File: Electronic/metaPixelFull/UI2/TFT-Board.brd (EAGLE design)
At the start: 56 x 60 mm, 28 parts, among them IC1 74HCT14N, IC2 74HCT14N

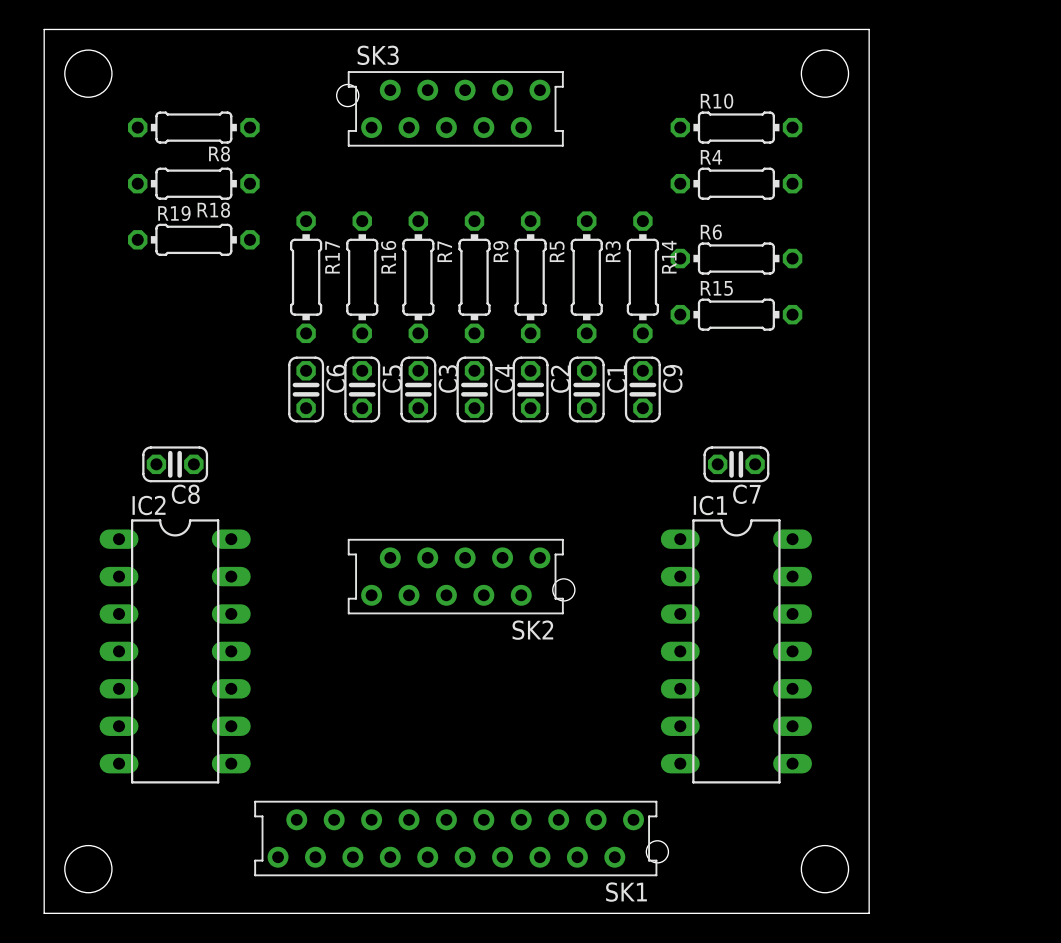
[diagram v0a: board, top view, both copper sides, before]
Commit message: rework UI
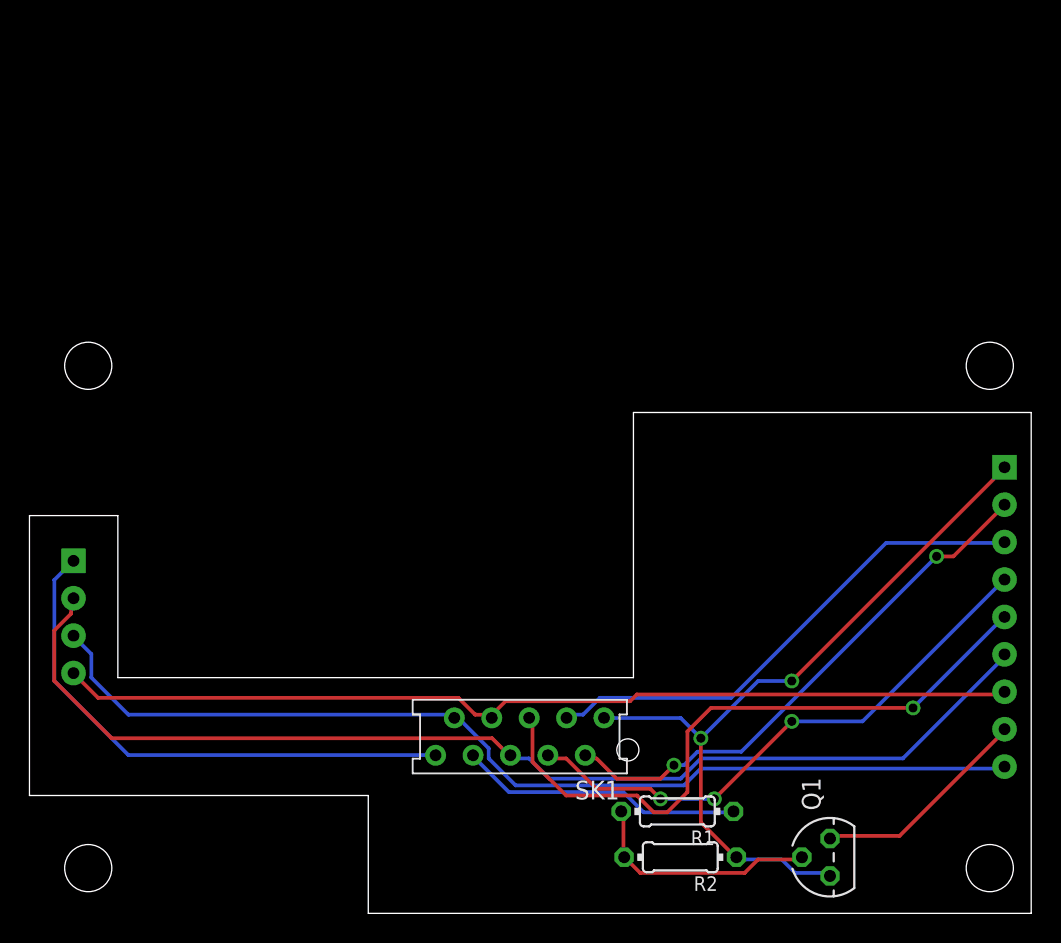
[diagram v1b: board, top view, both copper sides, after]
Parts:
- removed C1, C2, C3, C4, C5, C6, C7, C8, C9: .1µ, rcl:C025-024X044
- removed IC1, IC2: 74HCT14N, 74xx-eu:DIL14
- removed R10, R15, R4, R6, R8: 82k, resistor:0204/7
- removed R14, R3, R5, R7, R9: 15k, resistor:0204/7
- removed R16, R17, R18, R19: 10k, resistor:0204/7
- removed SK2: Display, jt-con-micromatch:AMP-215079-10
- removed SK3: (no value), jt-con-micromatch:AMP-215079-10
- added Q1: 2N3906, transistor-pnp:TO92
- added R1, R2: (no value), resistor:0204/7
- added U$1: 2.2_TFT_LCDNEW, 2.2"tft:2.2_TFT_LCD_LEDSEE
- SK1: value Host -> (none); device jt-con-micromatch:AMP-215079-20 -> jt-con-micromatch:AMP-215079-10
- moved SK1 7.20 mm to (38.0, 12.0)
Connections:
- removed net ENC1: C5.1, IC2.11, R16.2
- removed net ENC2: C6.1, IC2.13, R17.2
- removed net ENC_1: R16.1, R18.1, SK3.4
- removed net ENC_2: R17.1, R19.2, SK3.1
- removed net ENC_A: IC2.10, SK1.14
- removed net ENC_B: IC2.12, SK1.15
- removed net K1: C9.1, IC1.9, R14.2
- removed net K2: C1.1, IC1.11, R3.2
- removed net K3: C2.1, IC1.13, R5.2
- removed net K4: C3.1, IC1.3, R7.2
- removed net K5: C4.1, IC1.5, R9.2
- removed net KEY_1: IC1.8, SK1.1
- removed net KEY_2: IC1.10, SK1.2
- removed net KEY_3: IC1.12, SK1.3
- removed net KEY_4: IC1.6, SK1.4
- removed net KEY_5: IC1.4, SK1.5
- removed net K_1: R14.1, R15.1, SK3.10
- removed net K_2: R3.1, R4.1, SK3.7
- removed net K_3: R5.1, R6.1, SK3.8
- removed net K_4: R10.1, R9.1, SK3.6
- removed net K_5: R7.1, R8.1, SK3.3
- new net BG_LED: Q1.1, U$1.P$8_LED
- new net N$1: Q1.2, R1.2, R2.2
- net !LCD_CS: now also SK1.3, U$1.P$3_CS; no longer SK1.6, SK2.3
- net !LCD_RST: now also SK1.4, U$1.P$2_RESET; no longer SK1.7, SK2.4
- net !MEM_CS: now also SK1.10, U$1.P$2_SD_CS; no longer SK1.13, SK2.10
- net +3.3V: now also Q1.3, R2.1, SK1.1, U$1.P$5_VCC; no longer C7.1, C8.1, IC1.14, IC2.14, R10.2, R15.2, R18.2, R19.1, R4.2, R6.2, R8.2, SK1.17, SK1.19, SK2.1, SK3.9
- net GND: now also SK1.2, U$1.P$4_GND; no longer C1.2, C2.2, C3.2, C4.2, C5.2, C6.2, C7.2, C8.2, C9.2, IC1.7, IC2.7, SK1.16, SK1.18, SK1.20, SK2.2, SK3.2
- net LCD_DC: now also SK1.5, U$1.P$1_DC; no longer SK1.8, SK2.5
- net LCD_LED: now also R1.1, SK1.8; no longer SK1.11, SK2.8
- net MISO: now also SK1.9, U$1.P$3_SD_MISO, U$1.P$9_MISO; no longer SK1.12, SK2.9
- net MOSI: now also SK1.6, U$1.P$1_SD_MOSI, U$1.P$6_MOSI; no longer SK1.9, SK2.6
- net SCLK: now also SK1.7, U$1.P$4_SD_SCK, U$1.P$7_SCK; no longer SK1.10, SK2.7
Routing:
- net MOSI: track 0.00 -> 77.0 mm
- net MISO: track 0.00 -> 69.6 mm
- net SCLK: track 0.00 -> 65.4 mm
- net +3.3V: track 0.00 -> 51.5 mm, vias 0 -> 2
- net LCD_DC: track 0.00 -> 44.6 mm, vias 0 -> 1
- net !LCD_RST: track 0.00 -> 38.4 mm, vias 0 -> 3
- net GND: track 0.00 -> 36.9 mm, vias 0 -> 2
- net !MEM_CS: track 0.00 -> 36.7 mm
- net !LCD_CS: track 0.00 -> 34.7 mm
- net LCD_LED: track 0.00 -> 19.3 mm
- net N$1: track 0.00 -> 16.3 mm
- net BG_LED: track 0.00 -> 15.0 mm
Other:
- board size 56 x 60 mm -> 68 x 34 mm

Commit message: Sülzfleisch in Tüten
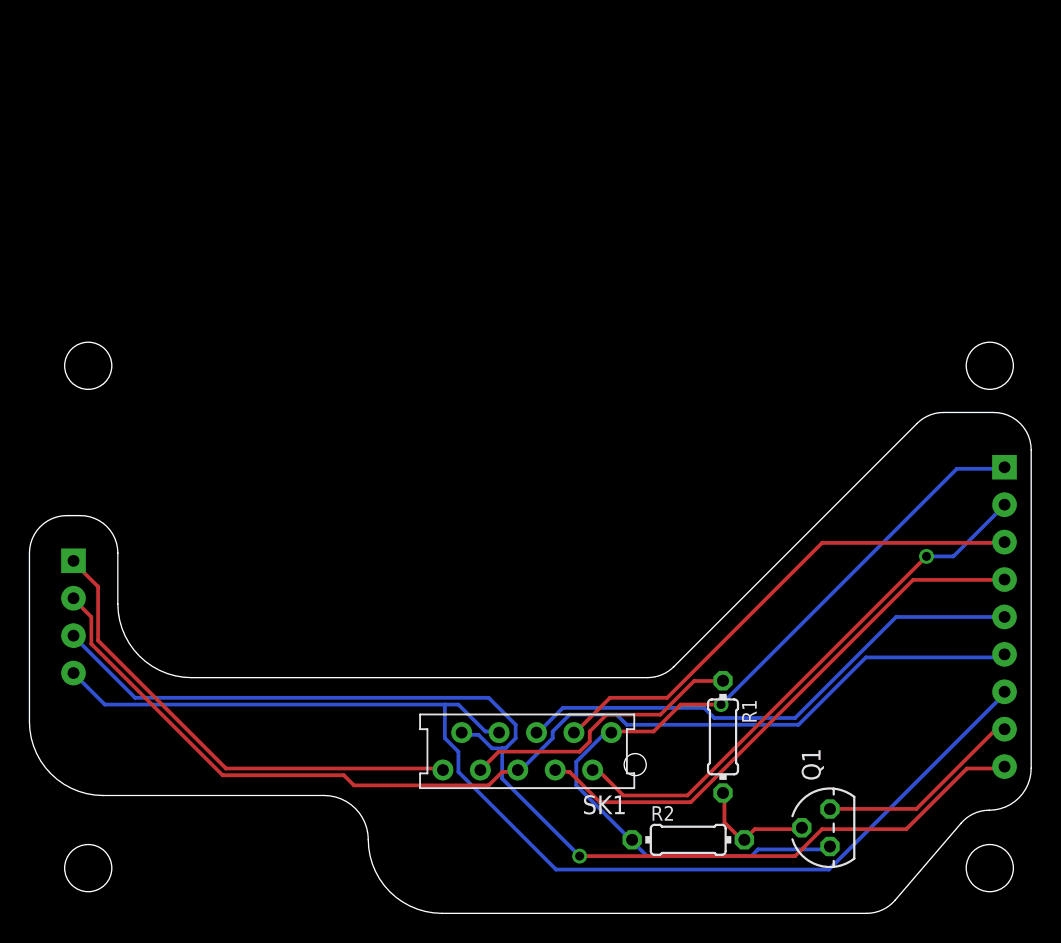
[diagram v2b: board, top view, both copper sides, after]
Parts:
- moved R1 5.93 mm to (46.1, 12.0), turned to 270 degrees
- moved Q1 2.00 mm to (53.3, 5.81)
- moved R2 1.30 mm to (43.7, 4.99), turned to 0 degrees
- moved SK1 1.12 mm to (38.5, 11.0)
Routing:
- net SCLK: track 65.4 -> 80.4 mm
- net MISO: track 69.6 -> 78.8 mm, vias 0 -> 1
- net LCD_DC: track 44.6 -> 35.6 mm, vias 1 -> 0
- net N$1: track 16.3 -> 8.16 mm
- net +3.3V: track 51.5 -> 58.6 mm, vias 2 -> 1
- net !MEM_CS: track 36.7 -> 33.1 mm
- net MOSI: track 77.0 -> 74.3 mm
- net BG_LED: track 15.0 -> 14.1 mm
- net !LCD_RST: track 38.4 -> 37.7 mm, vias 3 -> 0
- net GND: vias 2 -> 1
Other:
- outline, holes or cut-outs redrawn
